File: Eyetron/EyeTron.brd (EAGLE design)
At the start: 100 x 63.5 mm, 40 parts, among them IC1 4093N, IC2 4093N, IC3 4093N, IC4 4077N

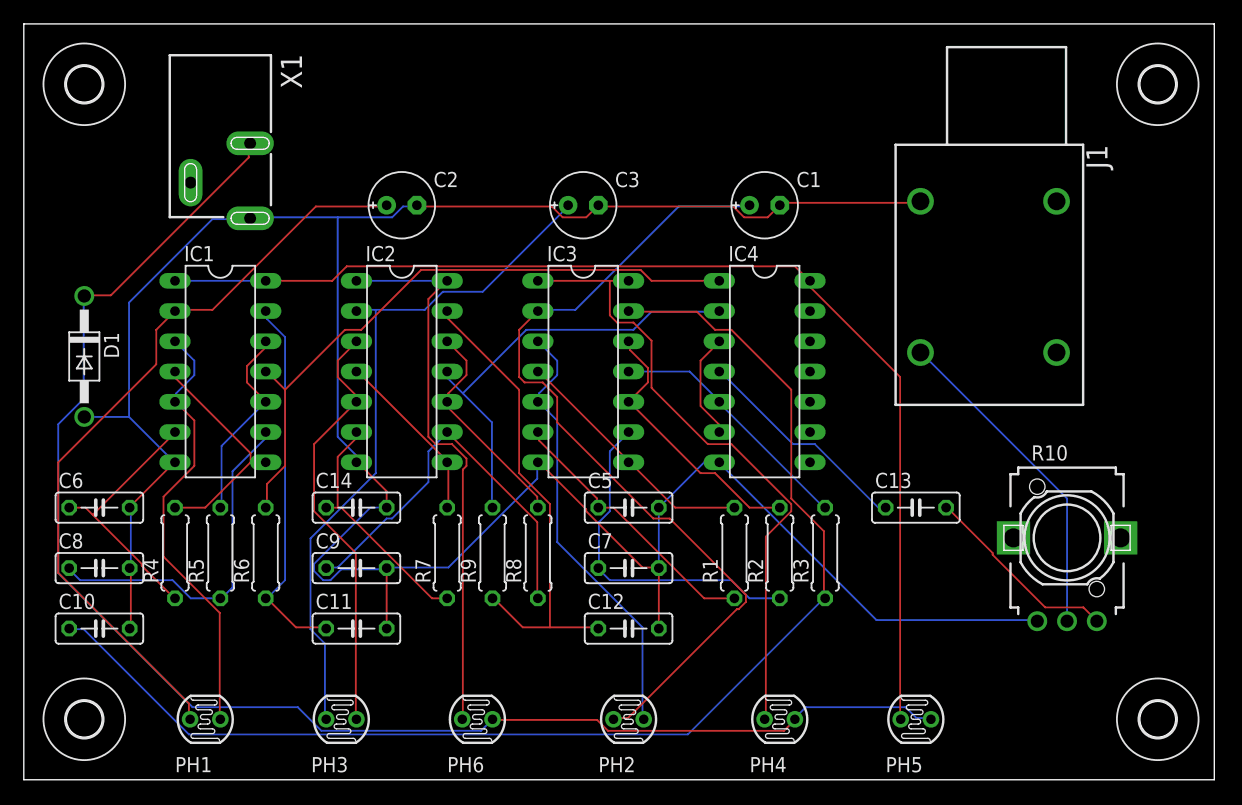
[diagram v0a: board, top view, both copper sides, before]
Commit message: Add files via upload
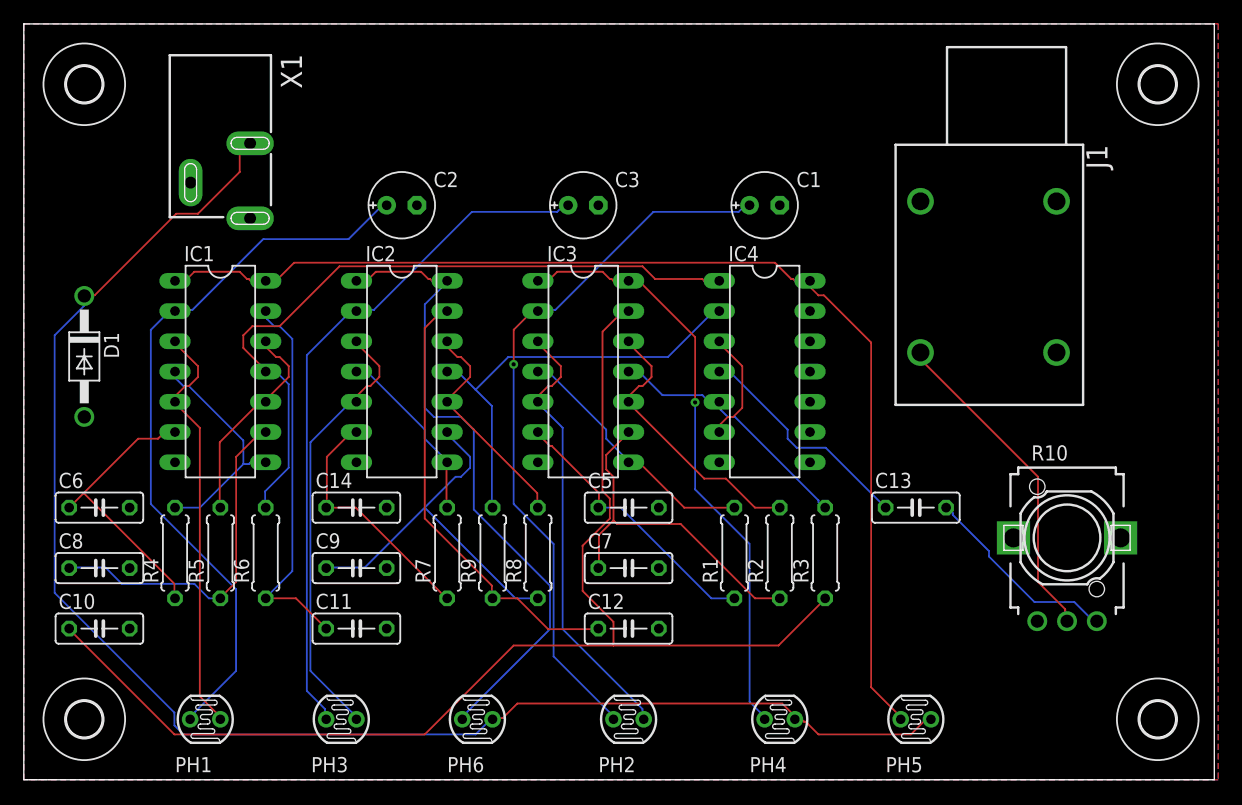
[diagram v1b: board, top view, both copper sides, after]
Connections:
- net N$34 renamed GND
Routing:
- net GND: track 233.6 -> 0.00 mm
- net N$14: track 71.5 -> 60.4 mm, vias 0 -> 1
- net N$29: track 47.4 -> 54.7 mm
- net N$1: track 53.9 -> 60.5 mm
- net N$21: track 107.1 -> 103.6 mm
- net N$20: track 53.7 -> 50.3 mm, vias 0 -> 1
- net N$30: track 125.0 -> 128.2 mm
- net N$15: track 64.5 -> 61.5 mm
- net N$28: track 40.1 -> 37.5 mm
- net N$4: track 36.8 -> 35.2 mm
- net N$23: track 21.9 -> 23.6 mm
- net N$27: track 33.6 -> 32.1 mm
- net N$22: track 94.4 -> 95.6 mm
- net N$5: track 36.0 -> 37.0 mm
- net N$19: track 28.8 -> 29.7 mm
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- added copper zone on layer 1, net GND
- added copper zone on layer 16, net GND
